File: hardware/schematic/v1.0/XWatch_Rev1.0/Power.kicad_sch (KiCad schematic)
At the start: 2 parts, among them IC1 DA9168, U4 MAX17048G_T10

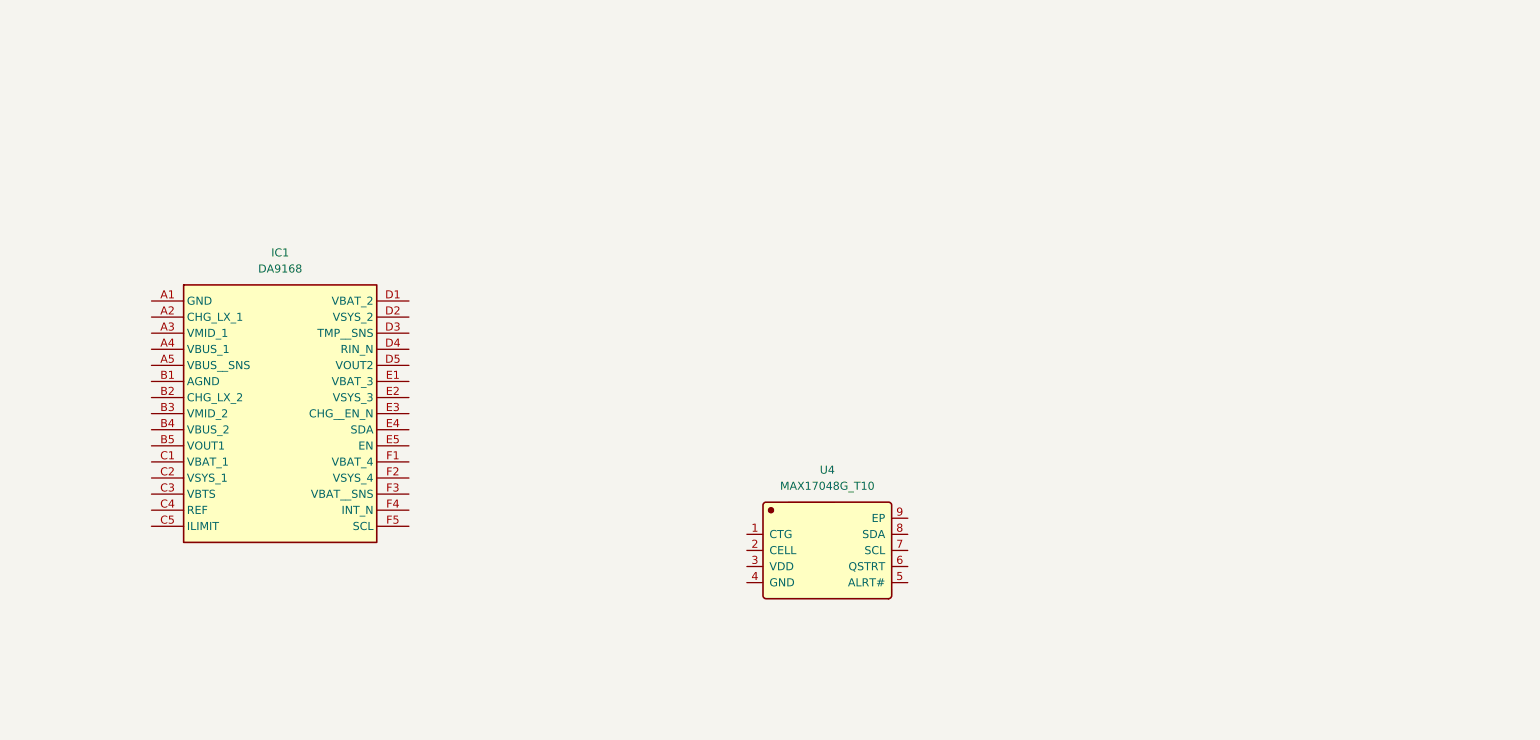
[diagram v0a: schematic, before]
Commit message: sch update
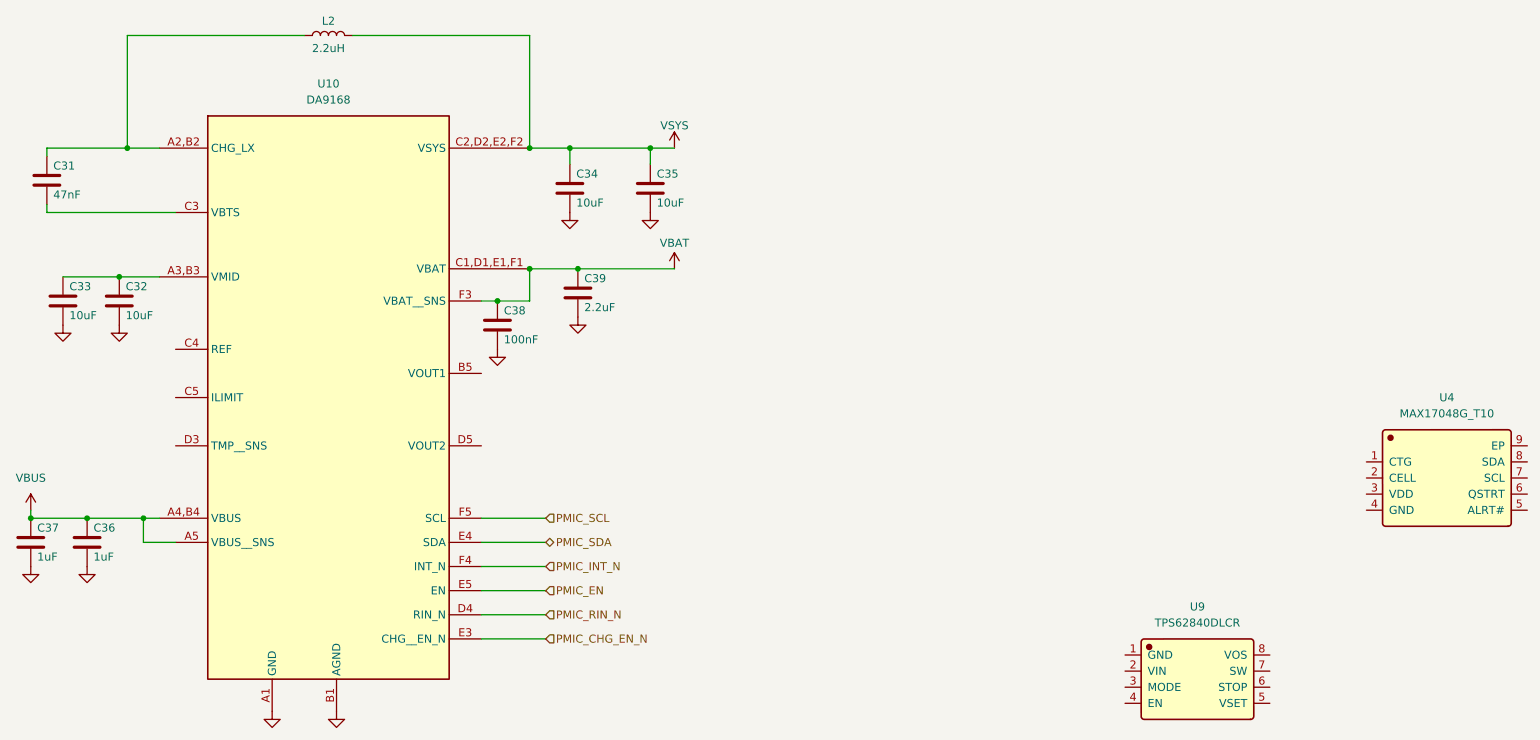
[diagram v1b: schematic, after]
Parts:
- removed IC1: DA9168, XWatch_Rev1.0:BGA30C40P5X6_214X254X56, symbol XWatch_Rev1.0:DA9168
- added C31: 47nF, XWatch_Rev1.0:GEN_C_0201, symbol XWatch_Rev1.0:C
- added C32, C33, C34, C35: 10uF, XWatch_Rev1.0:GEN_C_0402, symbol XWatch_Rev1.0:C
- added C36, C37: 1uF, XWatch_Rev1.0:GEN_C_0402, symbol XWatch_Rev1.0:C
- added C38: 100nF, XWatch_Rev1.0:GEN_C_0201, symbol XWatch_Rev1.0:C
- added C39: 2.2uF, XWatch_Rev1.0:GEN_C_0402, symbol XWatch_Rev1.0:C
- added L2: 2.2uH, XWatch_Rev1.0:L_0402_1005Metric, symbol XWatch_Rev1.0:L
- added U10: DA9168, symbol XWatch_Rev1.0:DA9168_1
- added U9: TPS62840DLCR, XWatch_Rev1.0:TPS62840DLCR, symbol XWatch_Rev1.0:TPS62840DLCR
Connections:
- new net: C31.1, L2.1, U10.A2,B2 (CHG_LX)
- new net: C31.2, U10.C3 (VBTS)
- new net: C32.1, C33.1, U10.A3,B3 (VMID)
- new net GND: C32.2, C33.2, C34.2, C35.2, C36.2, C37.2, C38.2, C39.2, U10.A1 (GND), U10.B1 (AGND)
- new net PMIC_CHG_EN_N: U10.E3 (CHG__EN_N)
- new net PMIC_EN: U10.E5 (EN)
- new net PMIC_INT_N: U10.F4 (INT_N)
- new net PMIC_RIN_N: U10.D4 (RIN_N)
- new net PMIC_SCL: U10.F5 (SCL)
- new net PMIC_SDA: U10.E4 (SDA)
- new net VBAT: C38.1, C39.1, U10.C1,D1,E1,F1 (VBAT), U10.F3 (VBAT__SNS)
- new net VBUS: C36.1, C37.1, U10.A4,B4 (VBUS), U10.A5 (VBUS__SNS)
- new net VSYS: C34.1, C35.1, L2.2, U10.C2,D2,E2,F2 (VSYS)
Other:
- moved on the sheet: U4
